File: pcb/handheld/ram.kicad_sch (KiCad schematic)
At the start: 3 parts, among them U1201 IS61WV25616EDBLL-10TLI

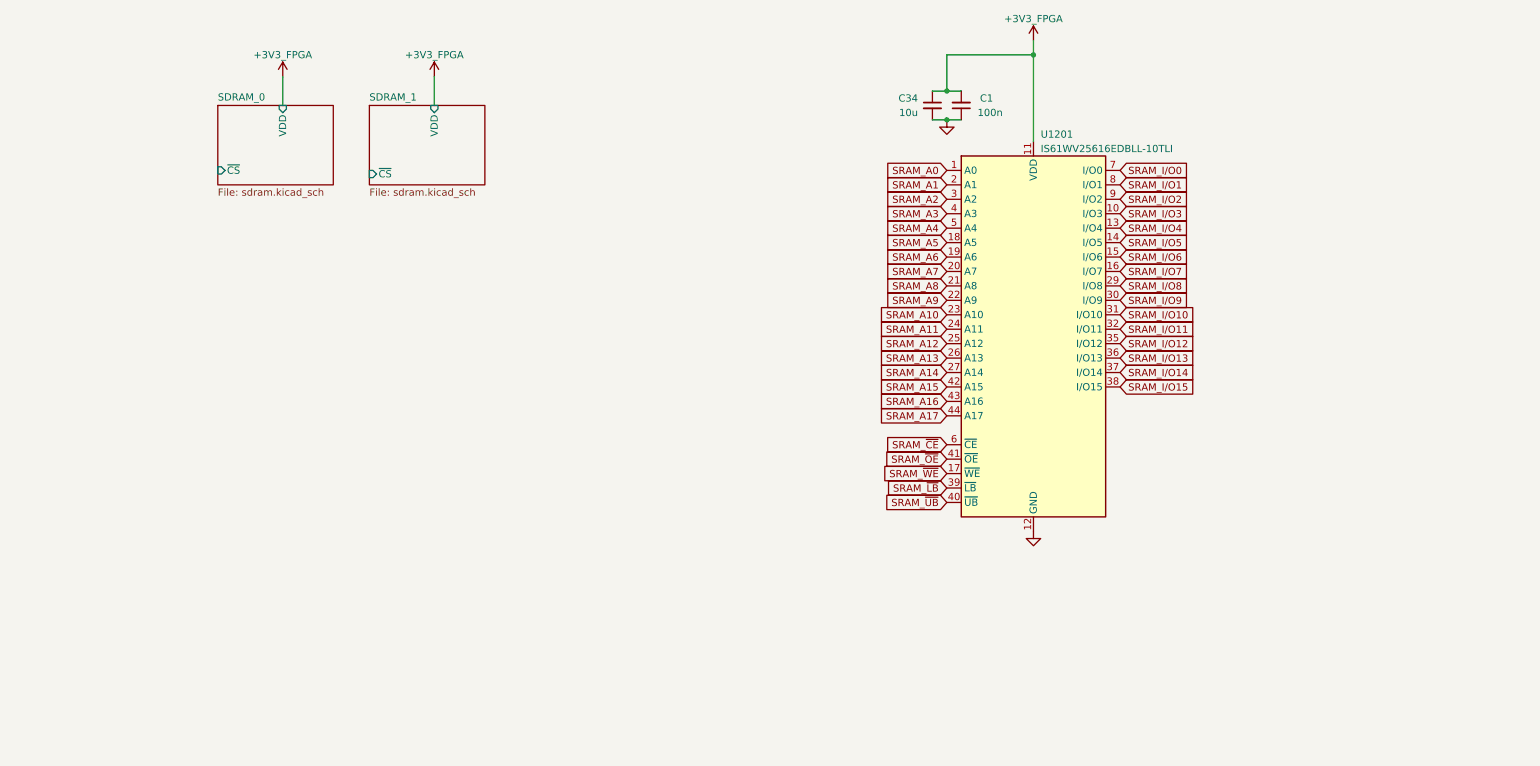
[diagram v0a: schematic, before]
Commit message: Rev A of PCB
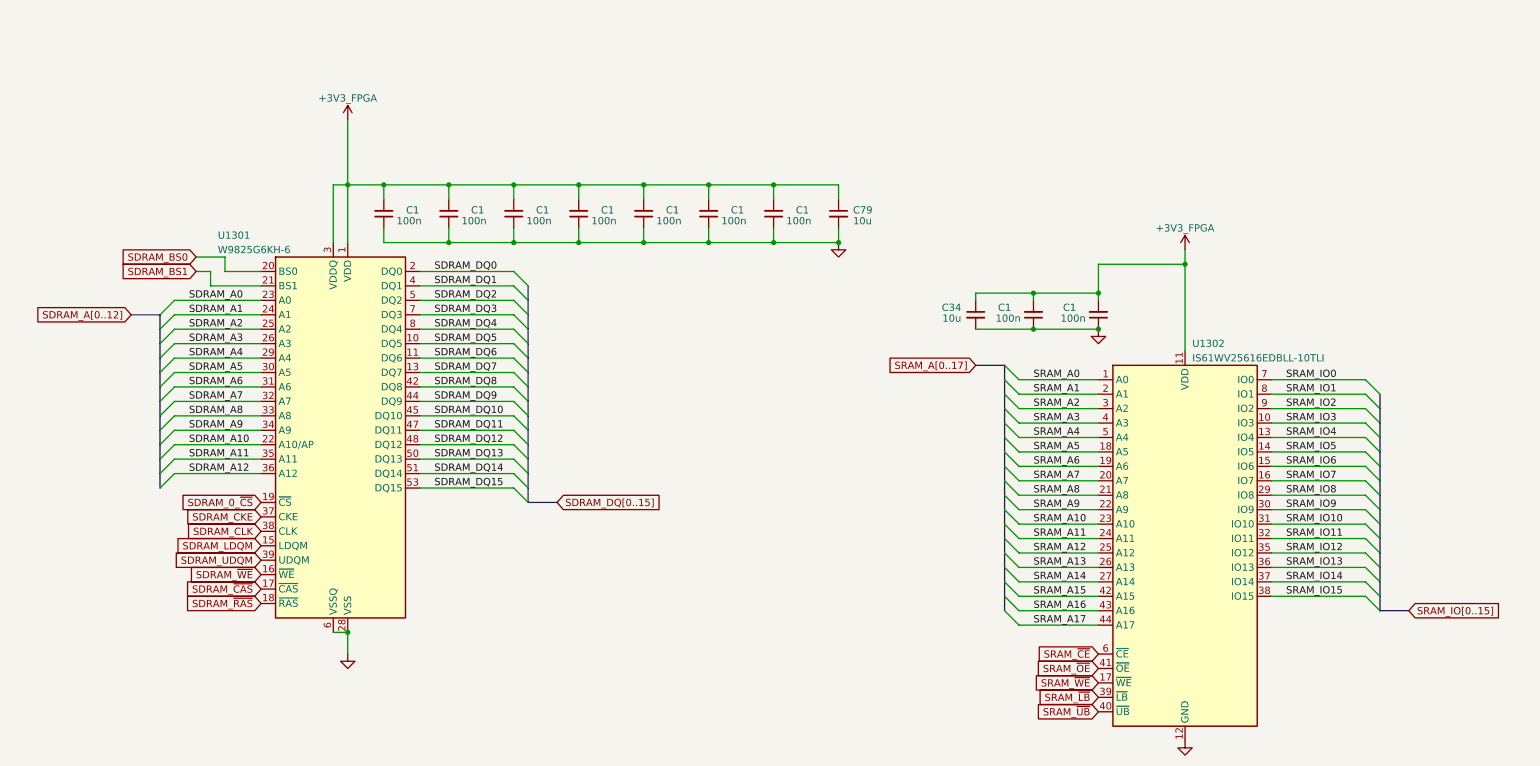
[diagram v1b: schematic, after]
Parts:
- added C1 (x8): 100n, Capacitor_SMD:C_0402_1005Metric, symbol Device:C_Small
- added C79: 10u, Capacitor_SMD:C_0402_1005Metric, symbol Device:C_Small
- added U1301: W9825G6KH-6, Package_SO:TSOP-II-54_22.2x10.16mm_P0.8mm, symbol Game_Bub:W9825G6KH-6
- renumbered U1201 to U1302
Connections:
- net +3V3_FPGA: now also C1.2, C1.2, C1.2, C1.2, C1.2, C1.2, C1.2, C1.2, C79.1, U1301.1 (VDD), U1301.14 (VDD), U1301.27 (VDD), U1301.3 (VDDQ), U1301.43 (VDDQ), U1301.49 (VDDQ), U1301.9 (VDDQ)
- net GND: now also C1.1, C1.1, C1.1, C1.1, C1.1, C1.1, C1.1, C1.1, C79.2, U1301.12 (VSSQ), U1301.28 (VSS), U1301.41 (VSS), U1301.46 (VSSQ), U1301.52 (VSSQ), U1301.54 (VSS), U1301.6 (VSSQ)
- net SRAM_I/O0 renamed SRAM_IO0
- net SRAM_I/O1 renamed SRAM_IO1
- net SRAM_I/O10 renamed SRAM_IO10
- net SRAM_I/O11 renamed SRAM_IO11
- net SRAM_I/O12 renamed SRAM_IO12
- net SRAM_I/O13 renamed SRAM_IO13
- net SRAM_I/O14 renamed SRAM_IO14
- net SRAM_I/O15 renamed SRAM_IO15
- net SRAM_I/O2 renamed SRAM_IO2
- net SRAM_I/O3 renamed SRAM_IO3
- net SRAM_I/O4 renamed SRAM_IO4
- net SRAM_I/O5 renamed SRAM_IO5
- net SRAM_I/O6 renamed SRAM_IO6
- net SRAM_I/O7 renamed SRAM_IO7
- net SRAM_I/O8 renamed SRAM_IO8
- net SRAM_I/O9 renamed SRAM_IO9
- new net SDRAM_0_~{CS}: U1301.19 (~{CS})
- new net SDRAM_A0: U1301.23 (A0)
- new net SDRAM_A1: U1301.24 (A1)
- new net SDRAM_A10: U1301.22 (A10/AP)
- new net SDRAM_A11: U1301.35 (A11)
- new net SDRAM_A12: U1301.36 (A12)
- new net SDRAM_A2: U1301.25 (A2)
- new net SDRAM_A3: U1301.26 (A3)
- new net SDRAM_A4: U1301.29 (A4)
- new net SDRAM_A5: U1301.30 (A5)
- new net SDRAM_A6: U1301.31 (A6)
- new net SDRAM_A7: U1301.32 (A7)
- new net SDRAM_A8: U1301.33 (A8)
- new net SDRAM_A9: U1301.34 (A9)
- new net SDRAM_BS0: U1301.20 (BS0)
- new net SDRAM_BS1: U1301.21 (BS1)
- new net SDRAM_CKE: U1301.37 (CKE)
- new net SDRAM_CLK: U1301.38 (CLK)
- new net SDRAM_DQ0: U1301.2 (DQ0)
- new net SDRAM_DQ1: U1301.4 (DQ1)
- new net SDRAM_DQ10: U1301.45 (DQ10)
- new net SDRAM_DQ11: U1301.47 (DQ11)
- new net SDRAM_DQ12: U1301.48 (DQ12)
- new net SDRAM_DQ13: U1301.50 (DQ13)
- new net SDRAM_DQ14: U1301.51 (DQ14)
- new net SDRAM_DQ15: U1301.53 (DQ15)
- new net SDRAM_DQ2: U1301.5 (DQ2)
- new net SDRAM_DQ3: U1301.7 (DQ3)
- new net SDRAM_DQ4: U1301.8 (DQ4)
- new net SDRAM_DQ5: U1301.10 (DQ5)
- new net SDRAM_DQ6: U1301.11 (DQ6)
- new net SDRAM_DQ7: U1301.13 (DQ7)
- new net SDRAM_DQ8: U1301.42 (DQ8)
- new net SDRAM_DQ9: U1301.44 (DQ9)
- new net SDRAM_LDQM: U1301.15 (LDQM)
- new net SDRAM_UDQM: U1301.39 (UDQM)
- new net SDRAM_~{CAS}: U1301.17 (~{CAS})
- new net SDRAM_~{RAS}: U1301.18 (~{RAS})
- new net SDRAM_~{WE}: U1301.16 (~{WE})
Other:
- removed sheet SDRAM_0
- removed sheet SDRAM_1
- moved on the sheet: C1, C34, U1302
